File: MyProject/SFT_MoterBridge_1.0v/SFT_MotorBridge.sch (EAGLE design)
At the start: 18 parts

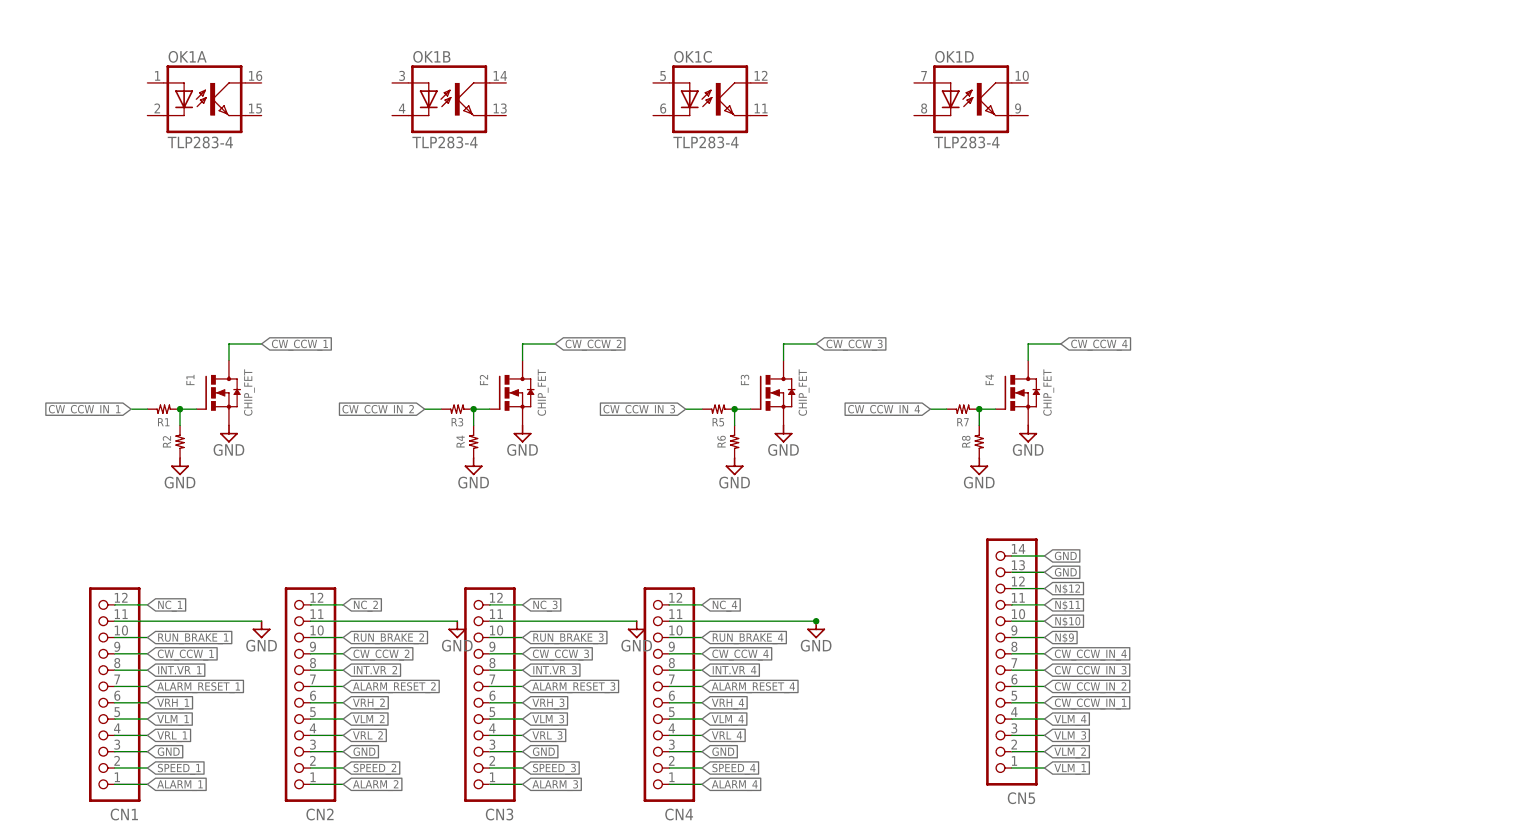
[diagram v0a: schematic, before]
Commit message: 月曜バイト行く前の更新
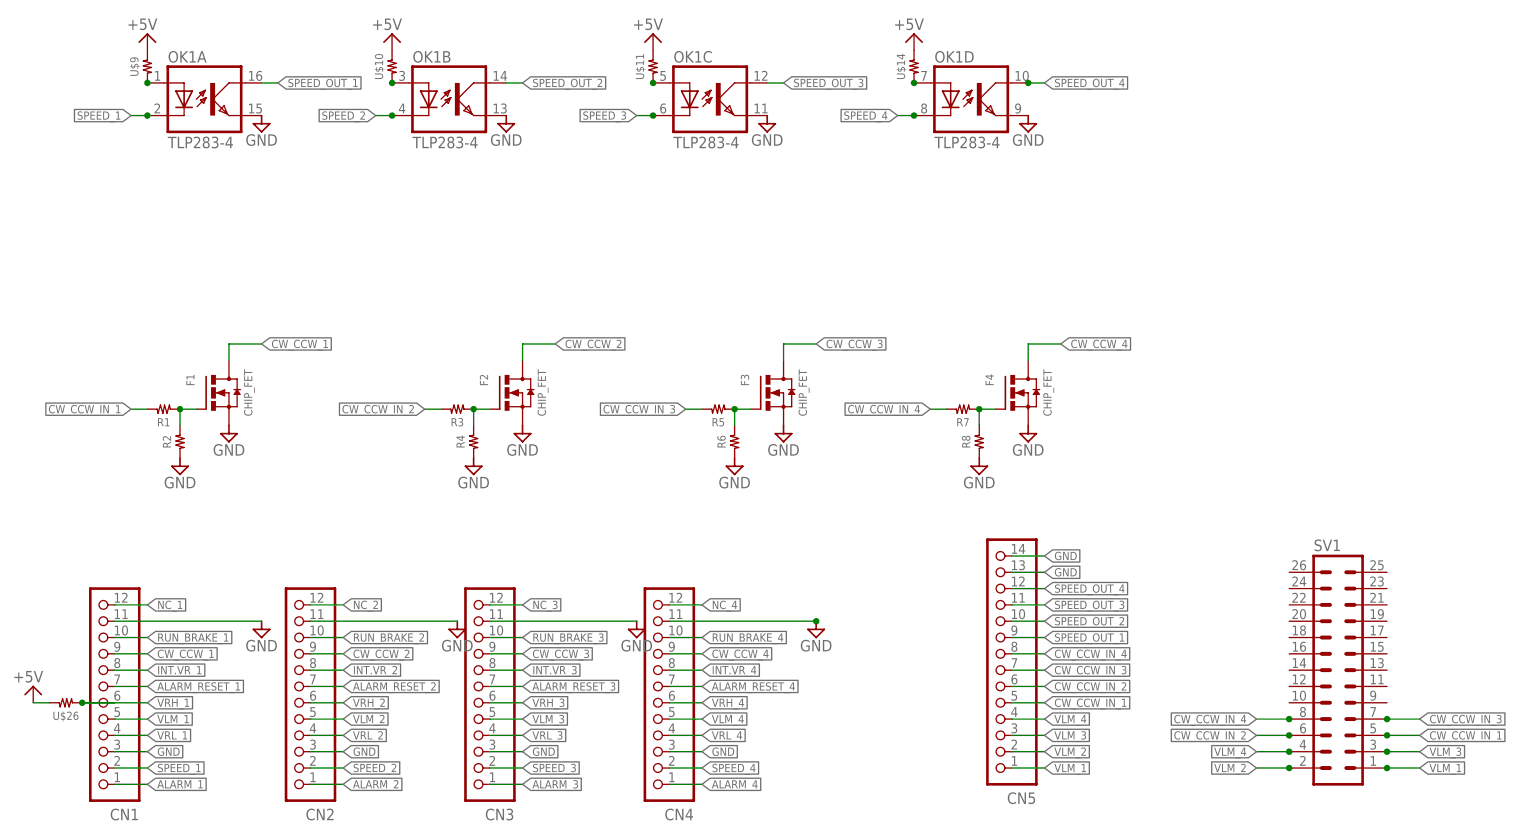
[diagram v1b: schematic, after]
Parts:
- added SV1: (no value), con-ml:ML26
- added U$10, U$11, U$14, U$26, U$9: (no value), 01_R:RESISTOR__SMD
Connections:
- removed net N$10: CN5.10
- removed net N$11: CN5.11
- removed net N$12: CN5.12
- removed net N$9: CN5.9
- new net +5V: U$10.P$2, U$11.P$2, U$14.P$2, U$26.P$2, U$9.P$2
- new net N$5: OK1A.A, U$9.P$1
- new net N$6: OK1B.A, U$10.P$1
- new net N$7: OK1C.A, U$11.P$1
- new net N$8: OK1D.A, U$14.P$1
- new net SPEED_OUT_1: CN5.9, OK1A.COL
- new net SPEED_OUT_2: CN5.10, OK1B.COL
- new net SPEED_OUT_3: CN5.11, OK1C.COL
- new net SPEED_OUT_4: CN5.12, OK1D.COL
- net CW_CCW_IN_1: now also SV1.5
- net CW_CCW_IN_2: now also SV1.6
- net CW_CCW_IN_3: now also SV1.7
- net CW_CCW_IN_4: now also SV1.8
- net GND: now also OK1A.EMIT, OK1B.EMIT, OK1C.EMIT, OK1D.EMIT
- net SPEED_1: now also OK1A.C
- net SPEED_2: now also OK1B.C
- net SPEED_3: now also OK1C.C
- net SPEED_4: now also OK1D.C
- net VLM_1: now also SV1.1
- net VLM_2: now also SV1.2
- net VLM_3: now also SV1.3
- net VLM_4: now also SV1.4
- net VRH_1: now also U$26.P$1
